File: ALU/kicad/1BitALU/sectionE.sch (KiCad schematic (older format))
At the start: 6 parts, among them U29 and6a, U30 inv6b, U31 and6b, U32 inv6c, U33 and6c, U34 or3d

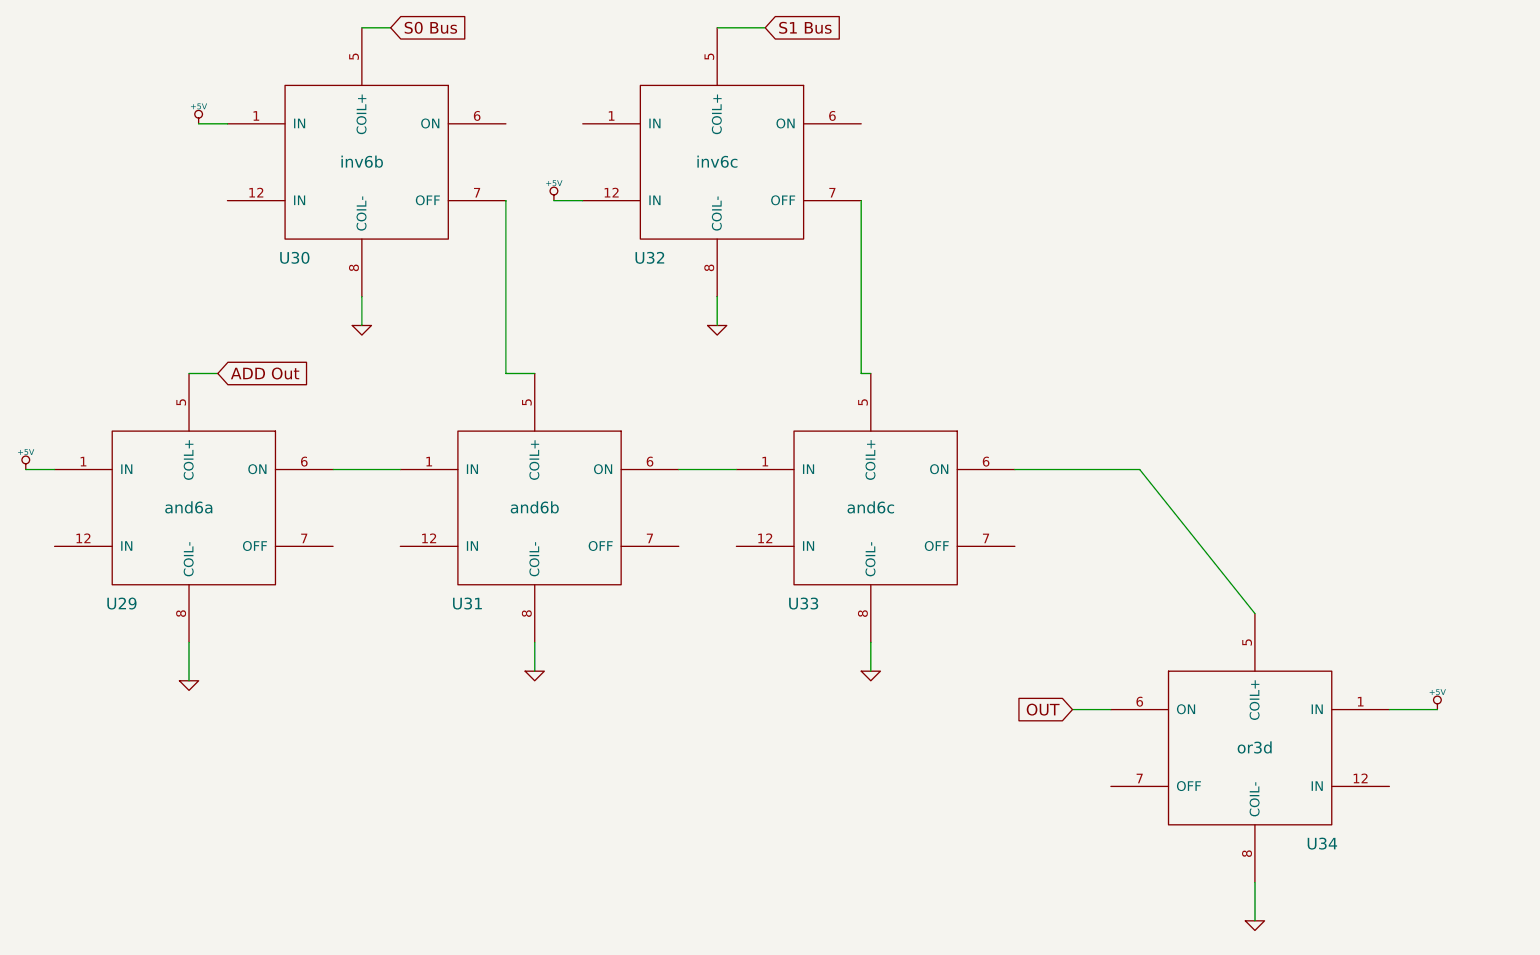
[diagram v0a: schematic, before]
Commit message: * improvements
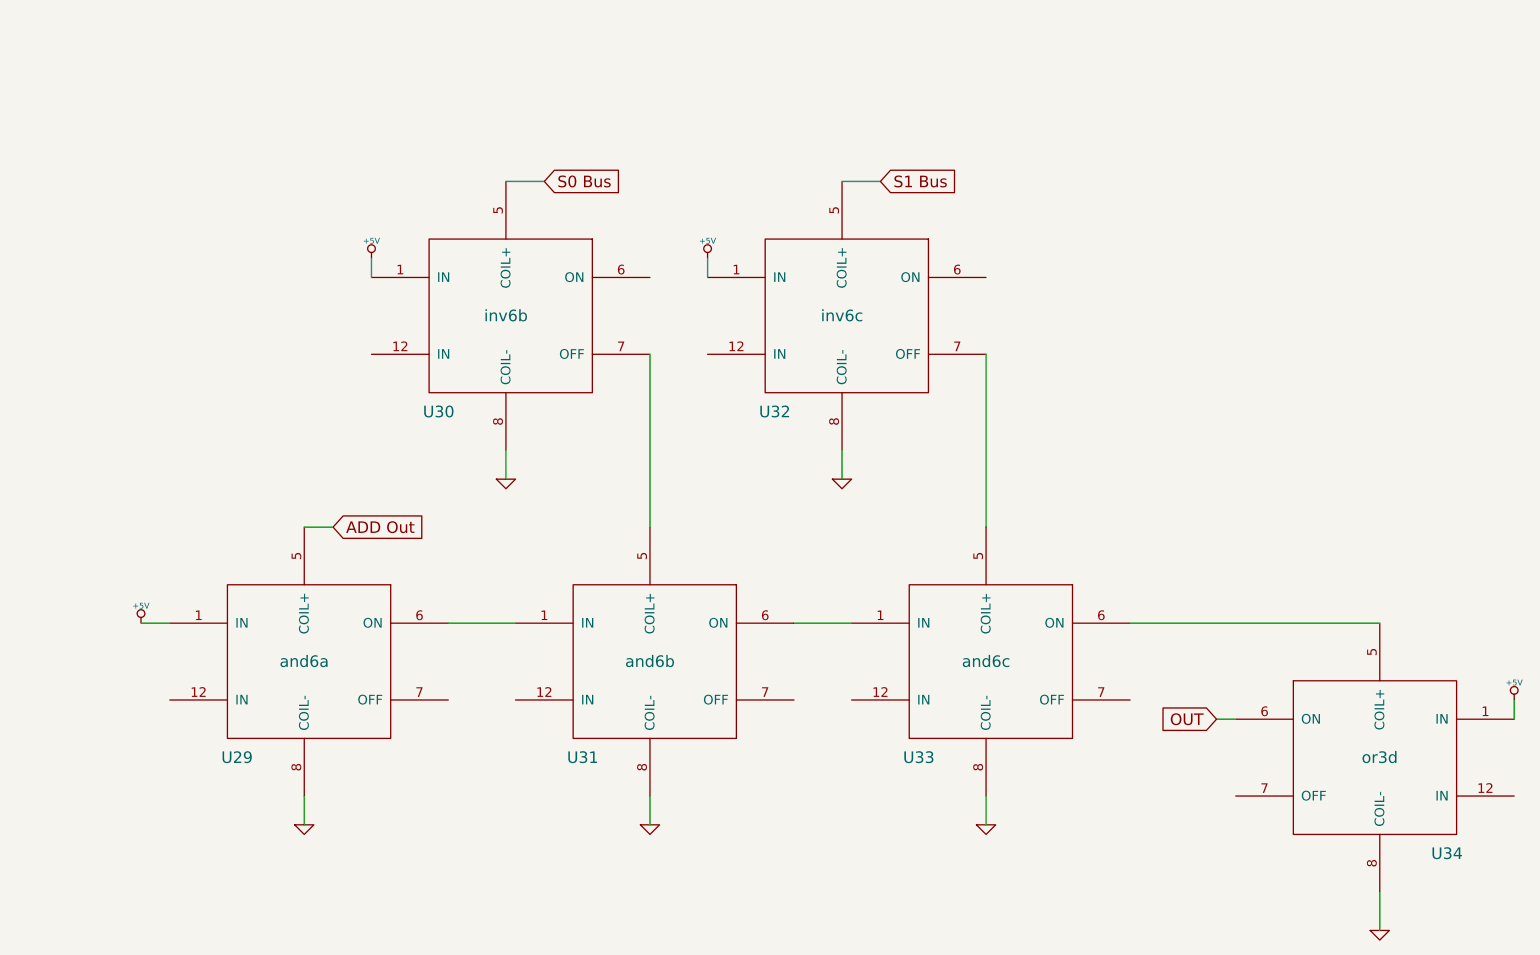
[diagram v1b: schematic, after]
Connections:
- net +5V: now also U32.1 (IN); no longer U32.12 (IN)
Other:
- moved on the sheet: U29, U30, U31, U32, U33, U34
